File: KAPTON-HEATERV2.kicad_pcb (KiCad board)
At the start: 2 copper layers, 90 x 90 mm, 32 parts, among them J1 XT60PW-M, J2 XT60PW-M, J3 1985276, J4 1985218, J5 10090926-P154XLF, K1 1-1393210-8, Q1 AO3400A, U1 TC4427ACOA, U2 INA181

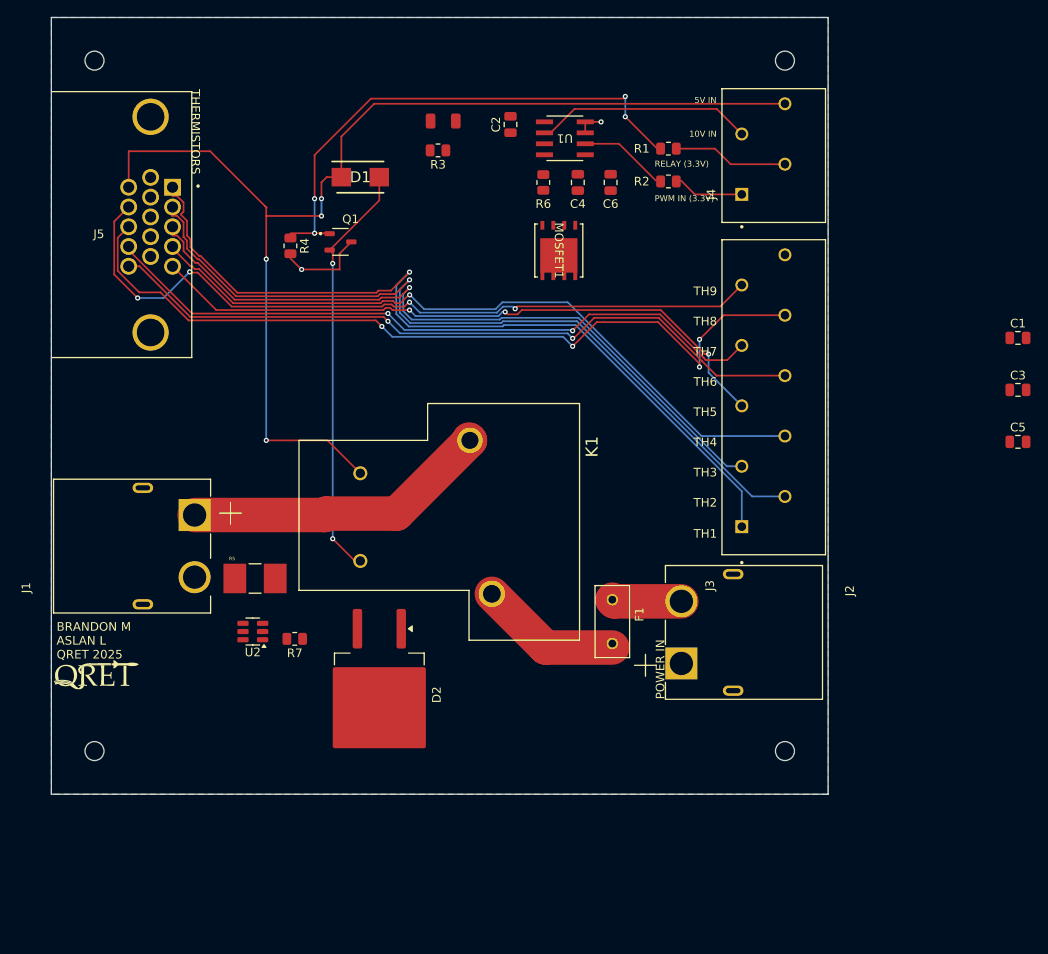
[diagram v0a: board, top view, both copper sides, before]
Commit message: started new one
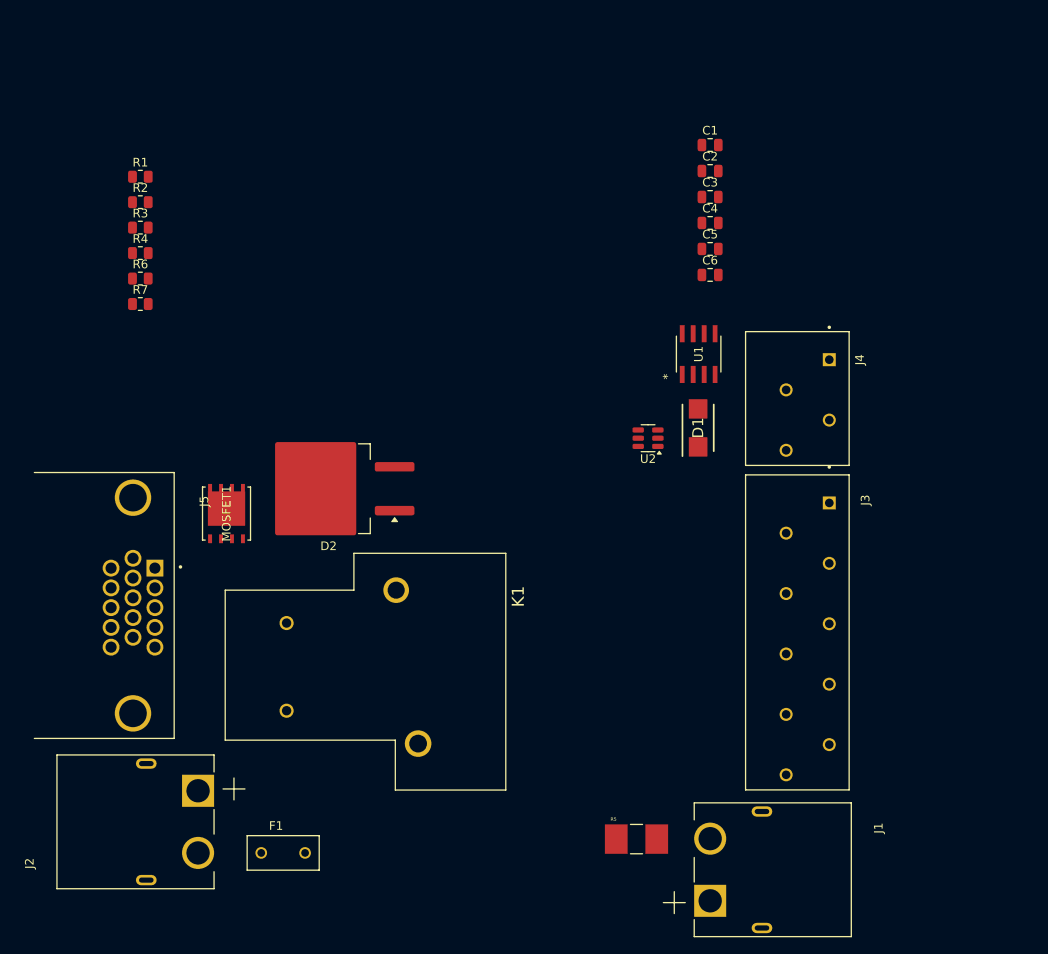
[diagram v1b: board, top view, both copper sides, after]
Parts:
- removed G***: LOGO, LOGO
- removed Q1: AO3400A, AO3400A (1):SOT95P280X125-3N
- removed the R5 at (73.6, 110.0)
- removed the R5 at (95.4, 57.0)
- removed REF** (x4): MountingHole_2.2mm_M2, MountingHole:MountingHole_2.2mm_M2
- added R5: R0.001, CRE2512_FZ_R001E_2 (1):RESC6432X90N, F.Cu at (117.8, 140.2)
- moved J1 80.9 mm to (132.3, 143.8), turned to -90 degrees
- moved J2 71.5 mm to (61.0, 138.2), turned to 90 degrees
- moved R1 61.3 mm to (60.3, 63.5), turned to 0 degrees
- moved R2 61.2 mm to (60.3, 66.4), turned to 0 degrees
- moved U2 51.0 mm to (119.1, 93.8)
- moved MOSFET1 49.1 mm to (70.3, 102.5), turned to 90 degrees
- moved D1 48.7 mm to (124.9, 92.5), turned to 90 degrees
- moved R6 48.0 mm to (60.3, 75.2), turned to 0 degrees
- moved F1 46.6 mm to (76.9, 141.8), turned to 0 degrees
- moved J5 44.2 mm to (59.5, 113.1)
- moved R7 42.7 mm to (60.3, 78.2), turned to 0 degrees
- moved C1 42.1 mm to (126.3, 59.8)
- moved C3 42.1 mm to (126.3, 65.8)
- moved C5 42.1 mm to (126.3, 71.8)
- moved R3 35.6 mm to (60.3, 69.3), turned to 0 degrees
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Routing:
- net 5V: track 133.1 -> 0.00 mm, vias 4 -> 0
- net TH1: track 95.2 -> 0.00 mm, vias 1 -> 0
- net TH8: track 94.5 -> 0.00 mm, vias 4 -> 0
- net TH2: track 92.6 -> 0.00 mm, vias 1 -> 0
- net TH9: track 87.7 -> 0.00 mm, vias 4 -> 0
- net TH6: track 83.3 -> 0.00 mm, vias 2 -> 0
- net TH3: track 82.6 -> 0.00 mm, vias 1 -> 0
- net TH4: track 82.0 -> 0.00 mm, vias 1 -> 0
- net TH7: track 79.0 -> 0.00 mm, vias 2 -> 0
- net TH5: track 74.9 -> 0.00 mm, vias 3 -> 0
- net Net-(Q1-Pad1): track 60.5 -> 0.00 mm, vias 4 -> 0
- net Net-(D1-A): track 48.7 -> 0.00 mm, vias 2 -> 0
- net /24V: track 35.6 -> 0.00 mm
- net 10V: track 25.2 -> 0.00 mm
- net (no net): track 17.0 -> 0.00 mm
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- removed copper zone on B.Cu, net GND
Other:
- board outline removed
- board text removed: "10V IN"
- board text removed: "5V IN"
- board text removed: "BRANDON M ASLAN L QRET 2025"
- board text removed: "POWER IN"
- board text removed: "PWM IN (3.3V)"
- board text removed: "RELAY (3.3V)"
- board text removed: "TH1"
- board text removed: "TH2"
- board text removed: "TH3"
- board text removed: "TH4"
- board text removed: "TH5"
- board text removed: "TH6"
- board text removed: "TH7"
- board text removed: "TH8"
- board text removed: "TH9"
- board text removed: "THERMISTORS"
